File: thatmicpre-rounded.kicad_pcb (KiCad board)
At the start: 2 copper layers, 45 x 24 mm, 12 parts, among them J1 Conn_01x07_Female, U1 THAT1512

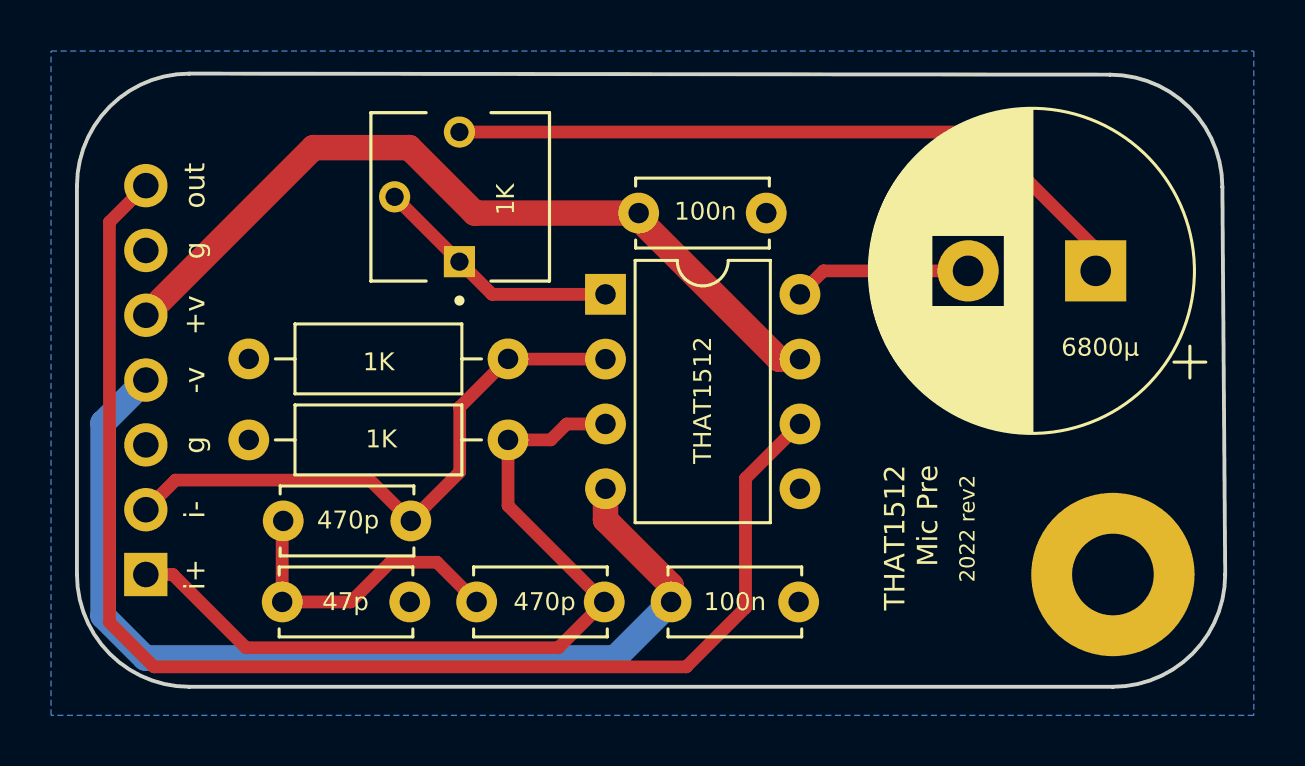
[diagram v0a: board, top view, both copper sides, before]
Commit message: rounded
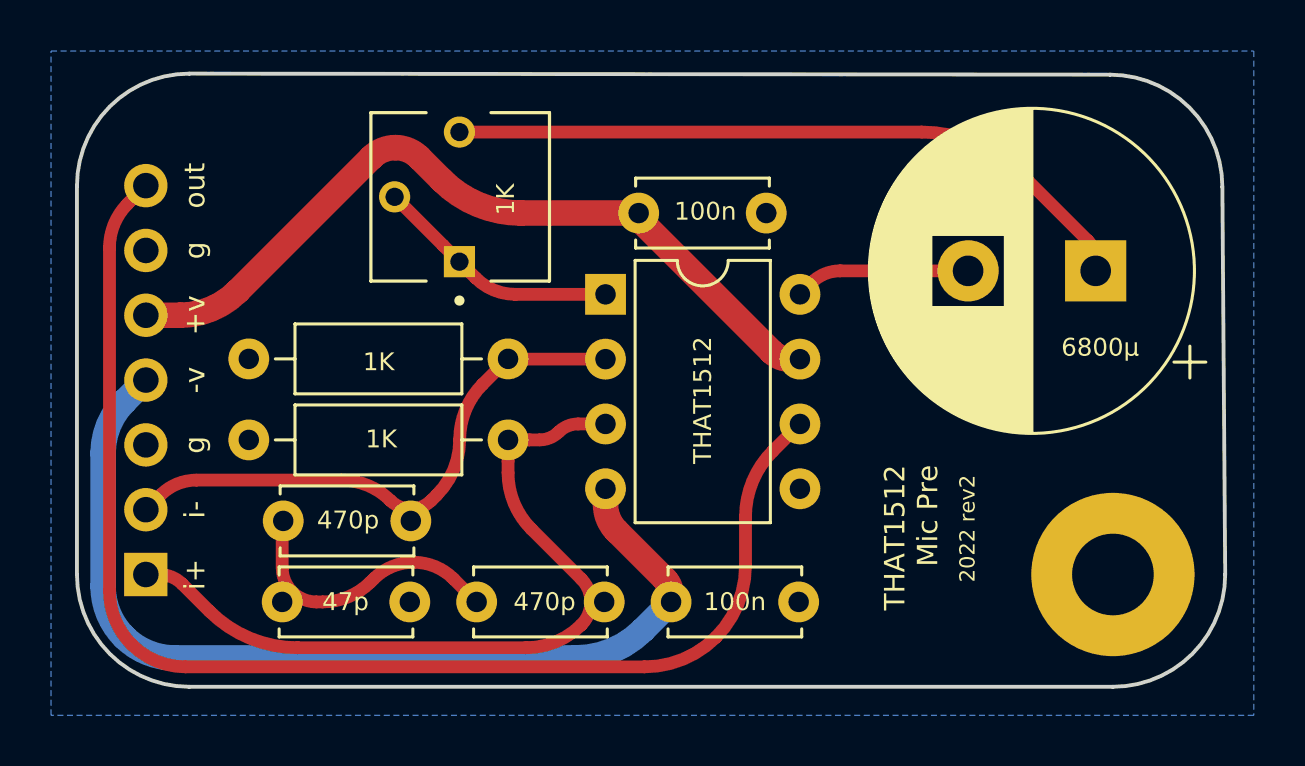
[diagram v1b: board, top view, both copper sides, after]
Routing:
- net +In: track 31.9 -> 30.2 mm
- net -In: track 23.3 -> 22.2 mm
- net Net-(C1-Pad1): track 12.1 -> 11.1 mm
- net Out: track 52.4 -> 51.4 mm
- net -15V: track 39.3 -> 38.6 mm
- net +15V: track 31.9 -> 31.3 mm
